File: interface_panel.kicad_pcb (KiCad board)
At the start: 2 copper layers, 48.5 x 32 mm, 7 parts, among them J1 Conn_02x04_Odd_Even

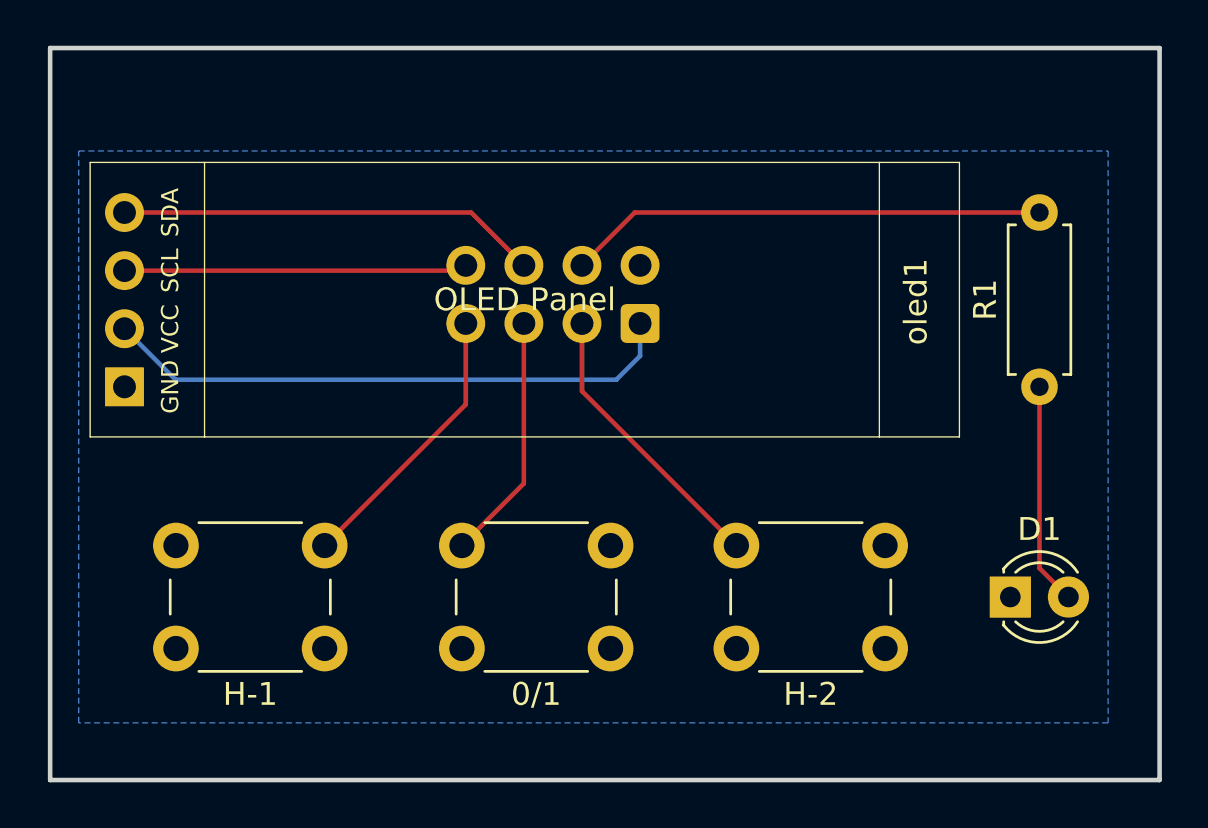
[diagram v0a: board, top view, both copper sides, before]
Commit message: panel_final
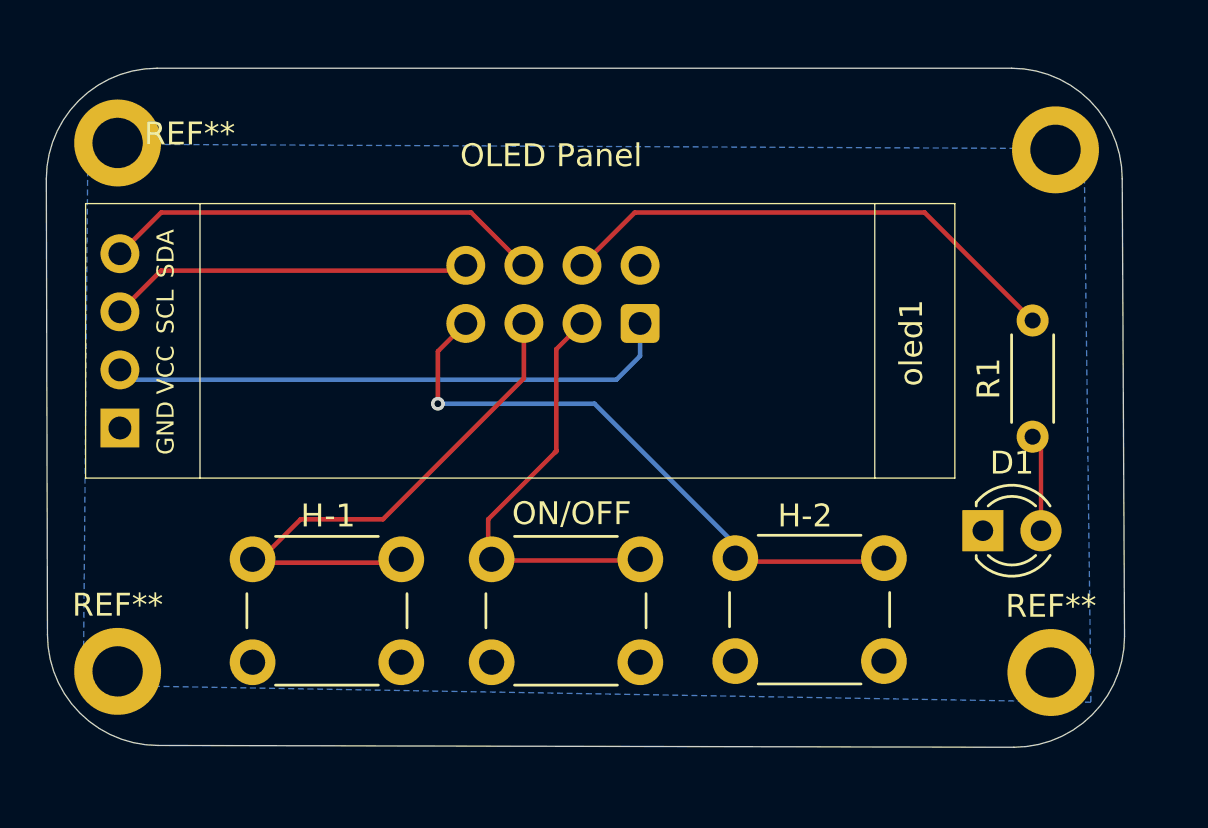
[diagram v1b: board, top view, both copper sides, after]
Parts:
- added REF**: MountingHole_2.2mm_M2_DIN965_Pad, MountingHole:MountingHole_2.2mm_M2_DIN965_Pad, F.Cu at (166.2, 64.0)
- added REF**: MountingHole_2.2mm_M2_DIN965_Pad, MountingHole:MountingHole_2.2mm_M2_DIN965_Pad, F.Cu at (125.2, 63.6)
- added REF**: MountingHole_2.2mm_M2_DIN965_Pad, MountingHole:MountingHole_2.2mm_M2_DIN965_Pad, F.Cu at (166.0, 86.8)
- added REF**: MountingHole_2.2mm_M2_DIN965_Pad, MountingHole:MountingHole_2.2mm_M2_DIN965_Pad, F.Cu at (125.2, 86.8)
- R1: footprint Resistor_THT:R_Axial_DIN0207_L6.3mm_D2.5mm_P7.62mm_Horizontal -> Resistor_THT:R_Axial_DIN0204_L3.6mm_D1.6mm_P5.08mm_Horizontal
- moved H-1 3.40 mm to (137.6, 86.3)
- moved D1 3.14 mm to (163.0, 80.6)
- moved R1 2.20 mm to (165.2, 76.5)
- moved oled1 1.81 mm to (161.8, 78.3)
- moved ON/OFF 1.43 mm to (148.1, 86.3)
- moved H-2 0.55 mm to (158.7, 86.3)
- renumbered 0/1 to ON/OFF
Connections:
- J1 pad 3: BT-2 -> BT-Pwr
- J1 pad 5: BT-Pwr -> BT-1
- J1 pad 7: BT-1 -> BT-2
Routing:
- net BT-2: track 12.5 -> 28.3 mm, vias 0 -> 1
- net BT-1: track 12.3 -> 24.2 mm
- net BT-Pwr: track 10.8 -> 18.7 mm
- net Net-(D1-A): track 9.71 -> 4.26 mm
- net S. LED: track 21.0 -> 22.6 mm
- net SCL: track 15.0 -> 16.0 mm
- net SDA: track 18.4 -> 19.4 mm
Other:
- board size 48.5 x 32 mm -> 47.1 x 29.7 mm
